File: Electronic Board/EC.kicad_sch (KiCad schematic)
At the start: 83 parts, among them J1 NMJ4HCD2, J2 4840.2201, J3 173950578, J4 NMJ4HCD2, J5 NMJ4HCD2, J6 NMJ4HCD2, J8 Conn_02x07_Odd_Even, SW2 SW_SPDT, U2 BU18SD2MG-MTR, U4 SGTL5000XNAA3, U5 IS42S16400J-xC, U502 BU33SD5WG-TR

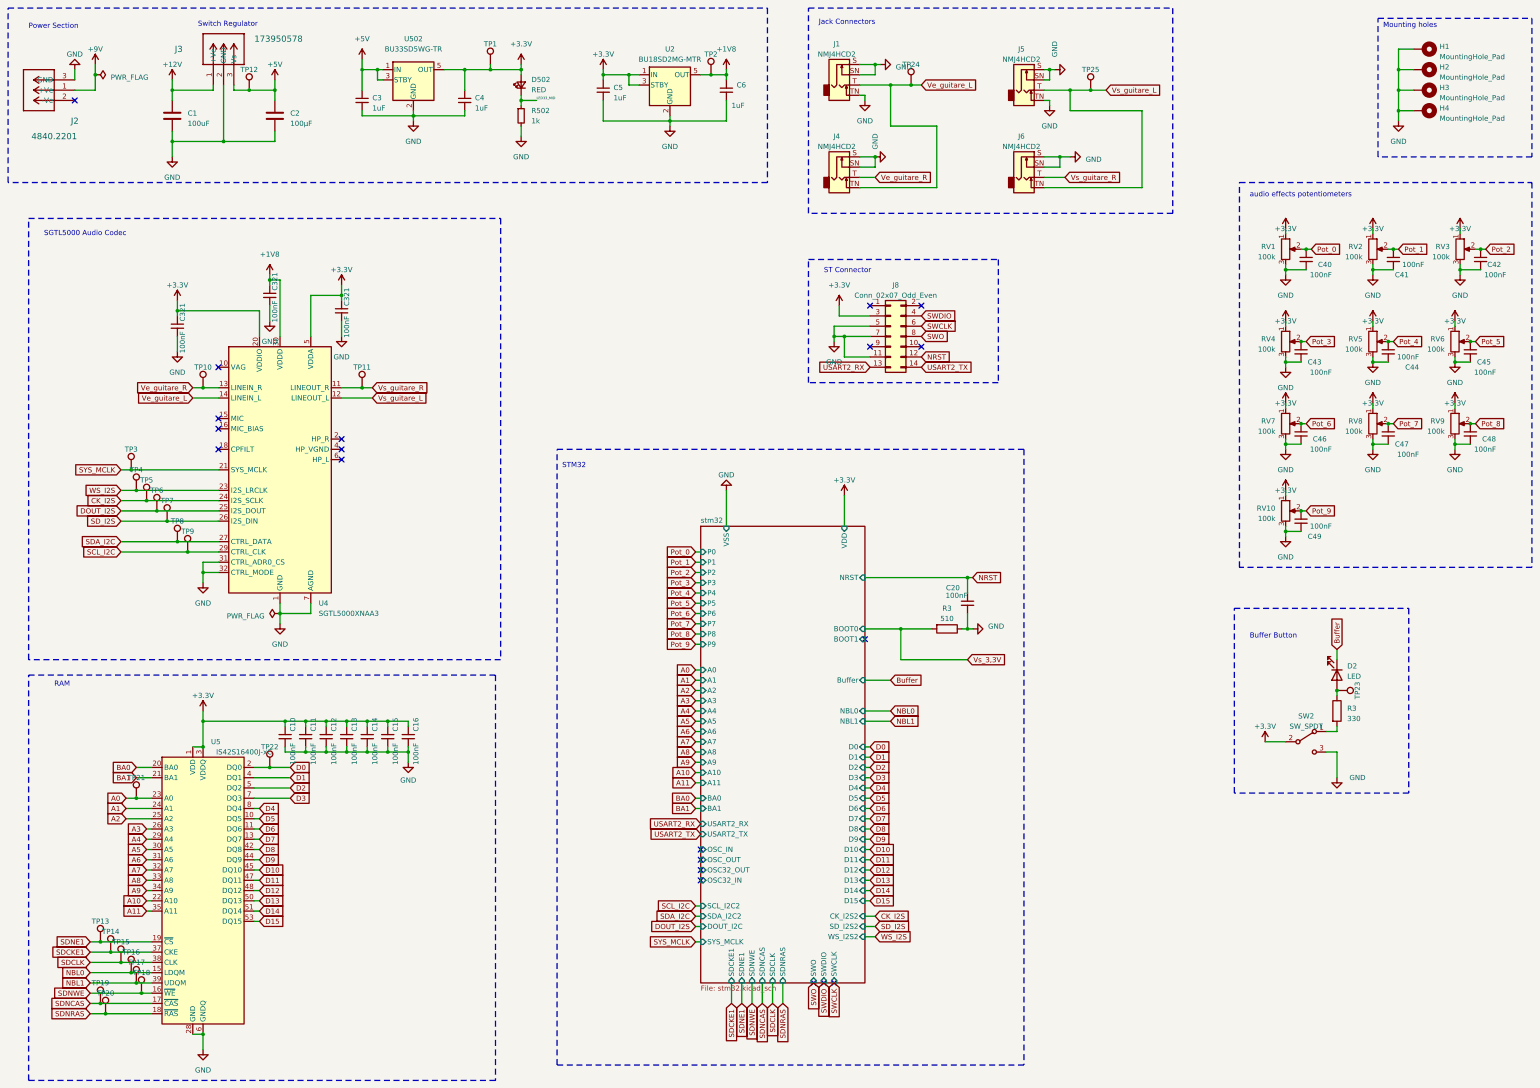
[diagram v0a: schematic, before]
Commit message: Add files via upload
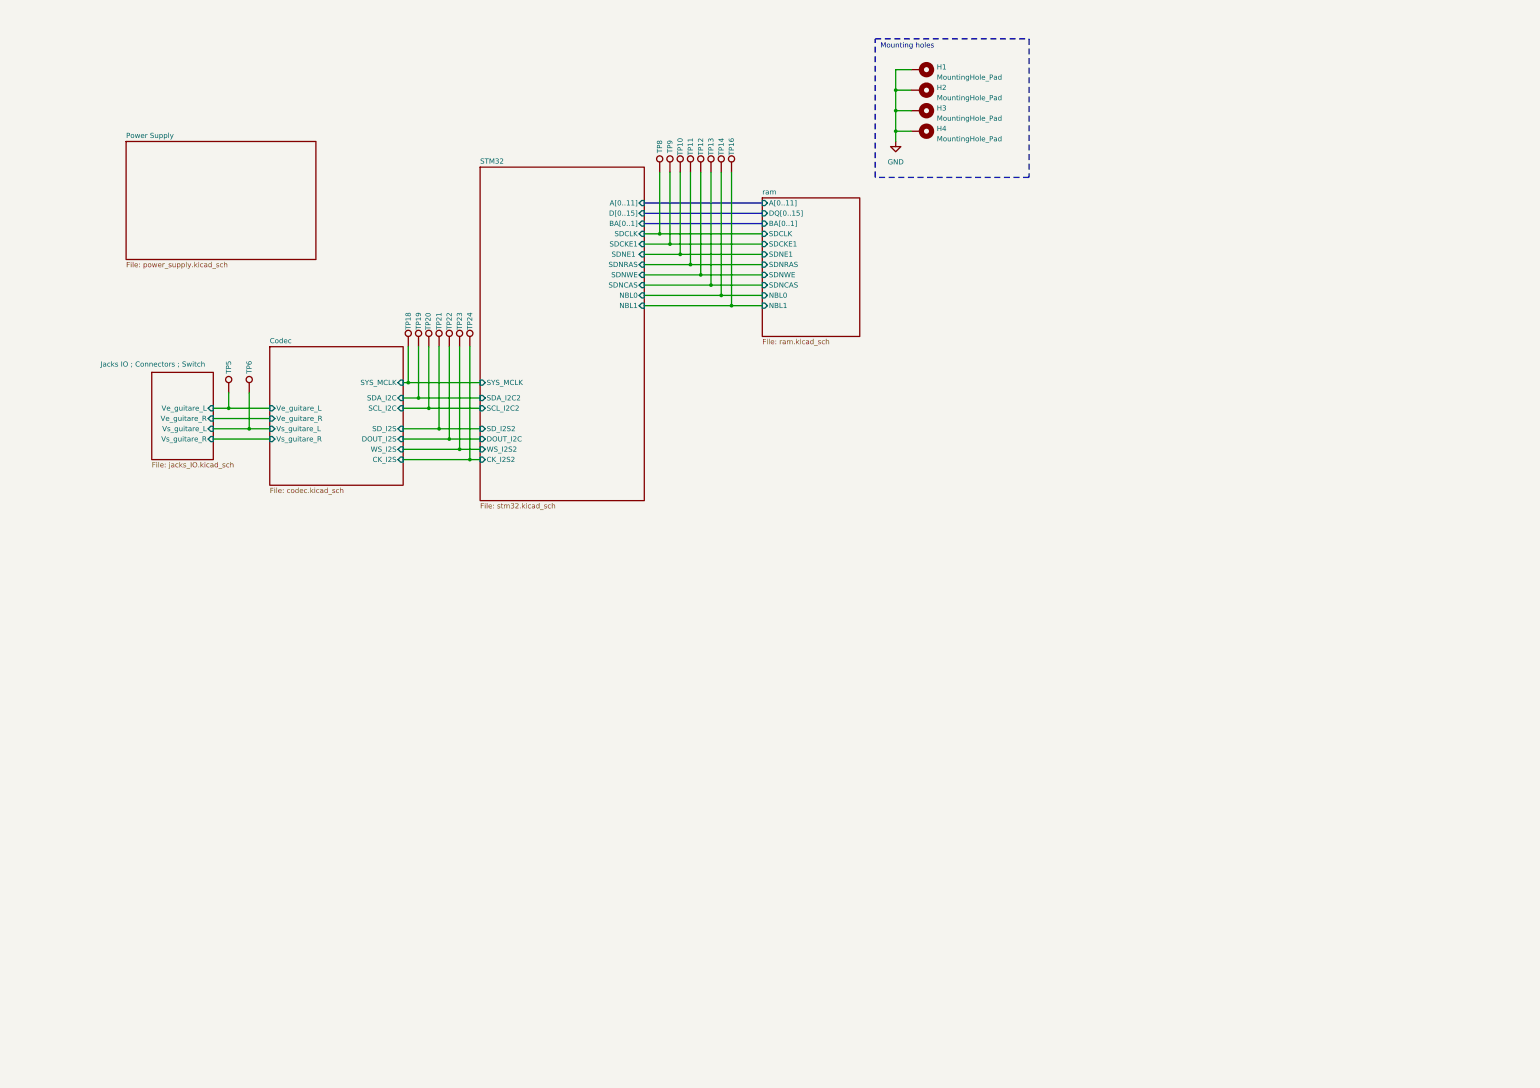
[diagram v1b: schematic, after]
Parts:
- removed C1: 100uF, Capacitor_SMD:C_0402_1005Metric_Pad0.74x0.62mm_HandSolder, symbol Device:C
- removed C10, C11, C12, C13, C14, C15, C16, C20, C321 (x3), C40, C41, C42, C43, C44, C45, C46, C47, C48, C49: 100nF, Capacitor_SMD:C_0402_1005Metric_Pad0.74x0.62mm_HandSolder, symbol Device:C_Small
- removed C2: 100µF, Capacitor_SMD:C_0402_1005Metric_Pad0.74x0.62mm_HandSolder, symbol Device:C
- removed C3, C4, C5, C6: 1uF, Capacitor_SMD:C_0402_1005Metric_Pad0.74x0.62mm_HandSolder, symbol Device:C_Small
- removed D2: LED, LED_SMD:LED_0402_1005Metric_Pad0.77x0.64mm_HandSolder, symbol Device:LED
- removed D502: RED, LED_SMD:LED_0402_1005Metric_Pad0.77x0.64mm_HandSolder, symbol Device:LED_Small
- removed J1, J4, J5, J6: NMJ4HCD2, Connector_Audio:Jack_6.35mm_Neutrik_NMJ4HCD2_Horizontal, symbol Connector_Audio:NMJ4HCD2
- removed J2: 4840.2201, Library:Regulator4840-2201, symbol REGULATEUR 5V:4840.2201
- removed J3: 173950578, Library:CONN3_950578_WRE_173950578, symbol Regulator 5V:173950578
- removed J8: Conn_02x07_Odd_Even, Connector_PinHeader_1.27mm:PinHeader_2x07_P1.27mm_Vertical_SMD, symbol Connector_Generic:Conn_02x07_Odd_Even
- removed R3: 510, Resistor_SMD:R_0201_0603Metric_Pad0.64x0.40mm_HandSolder, symbol Device:R
- removed R3: 330, Resistor_SMD:R_0201_0603Metric_Pad0.64x0.40mm_HandSolder, symbol Device:R
- removed R502: 1k, Resistor_SMD:R_0603_1608Metric, symbol Device:R_Small
- removed RV1, RV10, RV2, RV3, RV4, RV5, RV6, RV7, RV8, RV9: 100k, Library:Potentiometer_Alpha_RD901F-40-00D_Single_Vertical, symbol Device:R_Potentiometer
- removed SW2: SW_SPDT, Library:RS_Pro_SPDT_8466720, symbol Switch:SW_SPDT
- removed TP1, TP15, TP17, TP2, TP25, TP3, TP4, TP7: TestPoint, Connector_Pin:Pin_D1.1mm_L8.5mm_W2.5mm_FlatFork, symbol Connector:TestPoint
- removed U2: BU18SD2MG-MTR, Package_TO_SOT_SMD:SOT-23-5, symbol WITNS_ROHM:BU18SD2MG-MTR
- removed U4: SGTL5000XNAA3, Package_DFN_QFN:QFN-32-1EP_5x5mm_P0.5mm_EP3.6x3.6mm, symbol Audio:SGTL5000XNAA3
- removed U5: IS42S16400J-xC, Package_SO:TSOP-II-54_22.2x10.16mm_P0.8mm, symbol Memory_RAM:IS42S16400J-xC
- removed U502: BU33SD5WG-TR, Package_TO_SOT_SMD:SOT-23-5, symbol WITNS_ROHM:BU33SD5WG-TR
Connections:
- net Codec/WS_I2S: now reaches TP23.1
- net +5V renamed STM32/SDNWE
- net A0 renamed Codec/SD_I2S
- net CK_I2S renamed Codec/Ve_guitare_L
- net D0 renamed Codec/DOUT_I2S
- net DOUT_I2S renamed Codec/Vs_guitare_L
- net NBL0 renamed STM32/NBL1
- net SCL_I2C renamed STM32/SDCKE1
- net SDA_I2C renamed STM32/SDCLK
- net SDCKE1 renamed STM32/NBL0
- net SDNCAS renamed Codec/SDA_I2C
- net SDNE1 renamed STM32/SDNCAS
- net SDNRAS renamed Codec/SCL_I2C
- net SDNWE renamed Codec/SYS_MCLK
- net Ve_guitare_L renamed Codec/CK_I2S
- net Ve_guitare_R renamed STM32/SDNE1 
- net Vs_guitare_R renamed STM32/SDNRAS
- no-connect marks 20 -> 0
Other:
- sheet stm32 renamed STM32
- added sheet Codec (codec.kicad_sch)
- added sheet Jacks IO ; Connectors ; Switch (jacks_IO.kicad_sch)
- added sheet Power Supply (power_supply.kicad_sch)
- added sheet ram (ram.kicad_sch)
- sheet STM32 ports: added A[0..11], BA[0..1], D[0..15]; removed A0, A1, A10, A11, A2, A3, A4, A5, A6, A7, A8, A9, BA0, BA1, BOOT0, BOOT1, Buffer, D0, D1, D10, D11, D12, D13, D14, D15, D2, D3, D4, D5, D6, D7, D8, D9, NRST, OSC32_IN, OSC32_OUT, OSC_IN, OSC_OUT, P0, P1, P2, P3, P4, P5, P6, P7, P8, P9, SWCLK, SWDIO, SWO, USART2_RX, USART2_TX, VDD, VSS
- note removed: "Buffer Button"
- note removed: "Jack Connectors"
- note removed: "Power Section"
- note removed: "RAM"
- note removed: "SGTL5000 Audio Codec"
- note removed: "ST Connector"
- note removed: "STM32"
- note removed: "Switch Regulator"
- note removed: "audio effects potentiometers"
- moved on the sheet: H1, H2, H3, H4
